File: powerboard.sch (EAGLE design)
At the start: 25 parts, among them IC1 ISL9122AIRNZ-T, U1 MCP73831T-2DCI/MC, U2 MIC826RYMT-TR

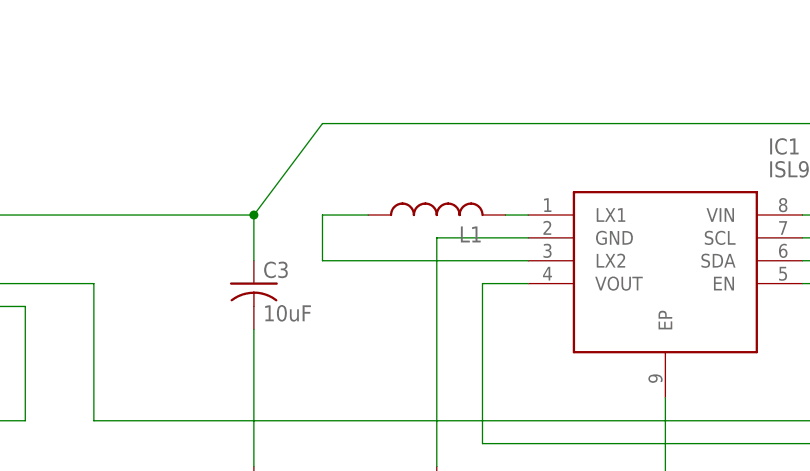
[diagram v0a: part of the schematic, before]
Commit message: progress
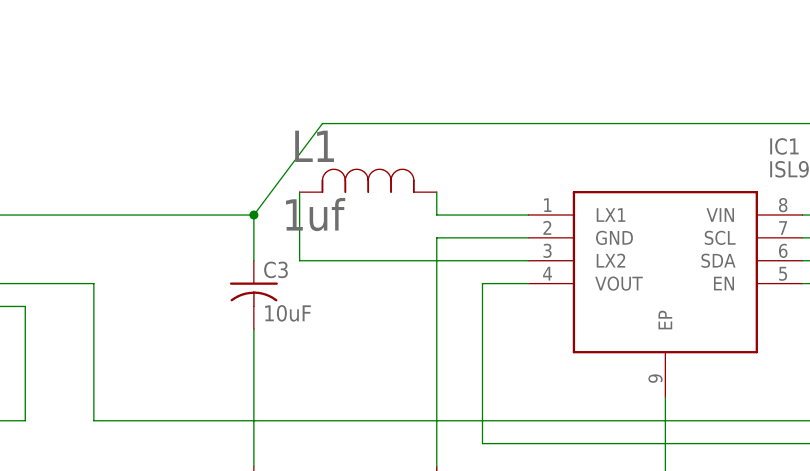
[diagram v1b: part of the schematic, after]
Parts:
- C1, C2, C3, C4: device rcl:C-USC0402 -> rcl:C-USC0603K
- L1: value (none) -> 1uf; device rcl:L-USL0201 -> vishayinductor:IHHP0806ZHER1R0M01
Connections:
- net INDUCTOR1: now also L1.2; no longer L1.1
- net INDUCTOR2: now also L1.1; no longer L1.2
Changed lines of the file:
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@@
 <part name="GND-IN" library="wirepad" library_urn="urn:adsk.eagle:library:412" deviceset="2,54/0,9" device="" package3d_urn="urn:adsk.eagle:package:30847/1"/>
 <part name="SUPPLY4" library="supply2" library_urn="urn:adsk.eagle:library:372" deviceset="GND" device=""/>
-<part name="C1" library="rcl" library_urn="urn:adsk.eagle:library:334" deviceset="C-US" device="C0402" package3d_urn="urn:adsk.eagle:package:23626/2" value="4.7uF"/>
-<part name="C2" library="rcl" library_urn="urn:adsk.eagle:library:334" deviceset="C-US" device="C0402" package3d_urn="urn:adsk.eagle:package:23626/2" value="4.7uF"/>
+<part name="C1" library="rcl" library_urn="urn:adsk.eagle:library:334" deviceset="C-US" device="C0603K" package3d_urn="urn:adsk.eagle:package:23680/2" value="4.7uF"/>
+<part name="C2" library="rcl" library_urn="urn:adsk.eagle:library:334" deviceset="C-US" device="C0603K" package3d_urn="urn:adsk.eagle:package:23680/2" value="4.7uF"/>
 <part name="SUPPLY5" library="supply2" library_urn="urn:adsk.eagle:library:372" deviceset="GND" device=""/>
 <part name="SUPPLY6" library="supply2" library_urn="urn:adsk.eagle:library:372" deviceset="GND" device=""/>
@@
 <part name="SUPPLY7" library="supply2" library_urn="urn:adsk.eagle:library:372" deviceset="GND" device=""/>
 <part name="IC1" library="ISL9122AIRNZ-T" deviceset="ISL9122AIRNZ-T" device=""/>
-<part name="C3" library="rcl" library_urn="urn:adsk.eagle:library:334" deviceset="C-US" device="C0402" package3d_urn="urn:adsk.eagle:package:23626/2" value="10uF"/>
+<part name="C3" library="rcl" library_urn="urn:adsk.eagle:library:334" deviceset="C-US" device="C0603K" package3d_urn="urn:adsk.eagle:package:23680/2" value="10uF"/>
 <part name="SUPPLY8" library="supply2" library_urn="urn:adsk.eagle:library:372" deviceset="GND" device=""/>
 <part name="SUPPLY9" library="supply2" library_urn="urn:adsk.eagle:library:372" deviceset="GND" device=""/>
-<part name="L1" library="rcl" library_urn="urn:adsk.eagle:library:334" deviceset="L-US" device="L0201" package3d_urn="urn:adsk.eagle:package:23513/2"/>
-<part name="C4" library="rcl" library_urn="urn:adsk.eagle:library:334" deviceset="C-US" device="C0402" package3d_urn="urn:adsk.eagle:package:23626/2" value="22uF"/>
+<part name="C4" library="rcl" library_urn="urn:adsk.eagle:library:334" deviceset="C-US" device="C0603K" package3d_urn="urn:adsk.eagle:package:23680/2" value="22uF"/>
 <part name="SUPPLY10" library="supply2" library_urn="urn:adsk.eagle:library:372" deviceset="GND" device=""/>
 <part name="SUPPLY11" library="supply2" library_urn="urn:adsk.eagle:library:372" deviceset="GND" device=""/>
@@
 <part name="3V3OUT" library="wirepad" library_urn="urn:adsk.eagle:library:412" deviceset="2,54/0,9" device="" package3d_urn="urn:adsk.eagle:package:30847/1"/>
 <part name="GNDOUT" library="wirepad" library_urn="urn:adsk.eagle:library:412" deviceset="2,54/0,9" device="" package3d_urn="urn:adsk.eagle:package:30847/1"/>
+<part name="L1" library="vishayinductor" deviceset="IHHP0806ZHER1R0M01" device="" value="1uf"/>
 </parts>
 <sheets>
@@
 <attribute name="VALUE" x="262.255" y="17.145" size="1.778" layer="96"/>
 </instance>
-<instance part="L1" gate="G$1" x="264.16" y="50.8" smashed="yes" rot="R90">
-<attribute name="NAME" x="269.24" y="49.53" size="1.778" layer="95" rot="R180"/>
-<attribute name="VALUE" x="269.24" y="54.61" size="1.778" layer="96" rot="R180"/>
-</instance>
 <instance part="C4" gate="G$1" x="327.66" y="45.72" smashed="yes">
 <attribute name="NAME" x="328.676" y="46.355" size="1.778" layer="95"/>
@@
 <attribute name="NAME" x="344.043" y="33.7058" size="1.778" layer="95" rot="R180"/>
 <attribute name="VALUE" x="333.883" y="36.322" size="1.778" layer="96" rot="R180"/>
+</instance>
+<instance part="L1" gate="A" x="248.92" y="53.34" smashed="yes">
+<attribute name="VALUE" x="246.9388" y="49.0728" size="3.4798" layer="96" ratio="10" rot="SR0"/>
+<attribute name="NAME" x="248.0056" y="56.6928" size="3.4798" layer="95" ratio="10" rot="SR0"/>
 </instance>
 </instances>
@@
 <segment>
 <pinref part="IC1" gate="G$1" pin="LX1"/>
-<pinref part="L1" gate="G$1" pin="2"/>
-<wire x1="271.78" y1="50.8" x2="274.32" y2="50.8" width="0.1524" layer="91"/>
+<wire x1="264.16" y1="50.8" x2="274.32" y2="50.8" width="0.1524" layer="91"/>
+<pinref part="L1" gate="A" pin="1"/>
+<wire x1="264.16" y1="53.34" x2="264.16" y2="50.8" width="0.1524" layer="91"/>
 </segment>
 </net>
 <net name="INDUCTOR1" class="1">
 <segment>
-<pinref part="L1" gate="G$1" pin="1"/>
-<wire x1="256.54" y1="50.8" x2="251.46" y2="50.8" width="0.1524" layer="91"/>
-<wire x1="251.46" y1="50.8" x2="251.46" y2="45.72" width="0.1524" layer="91"/>
 <pinref part="IC1" gate="G$1" pin="LX2"/>
-<wire x1="251.46" y1="45.72" x2="274.32" y2="45.72" width="0.1524" layer="91"/>
-</segment>
-</net>
+<wire x1="248.92" y1="53.34" x2="248.92" y2="45.72" width="0.1524" layer="91"/>
+<wire x1="248.92" y1="45.72" x2="274.32" y2="45.72" width="0.1524" layer="91"/>
+<pinref part="L1" gate="A" pin="2"/>
+</segment>
+</net>
